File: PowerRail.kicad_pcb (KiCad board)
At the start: 2 copper layers, 25.4 x 25.4 mm, 20 parts, among them P1 PIN, P2 POUT, U1 ADP5071

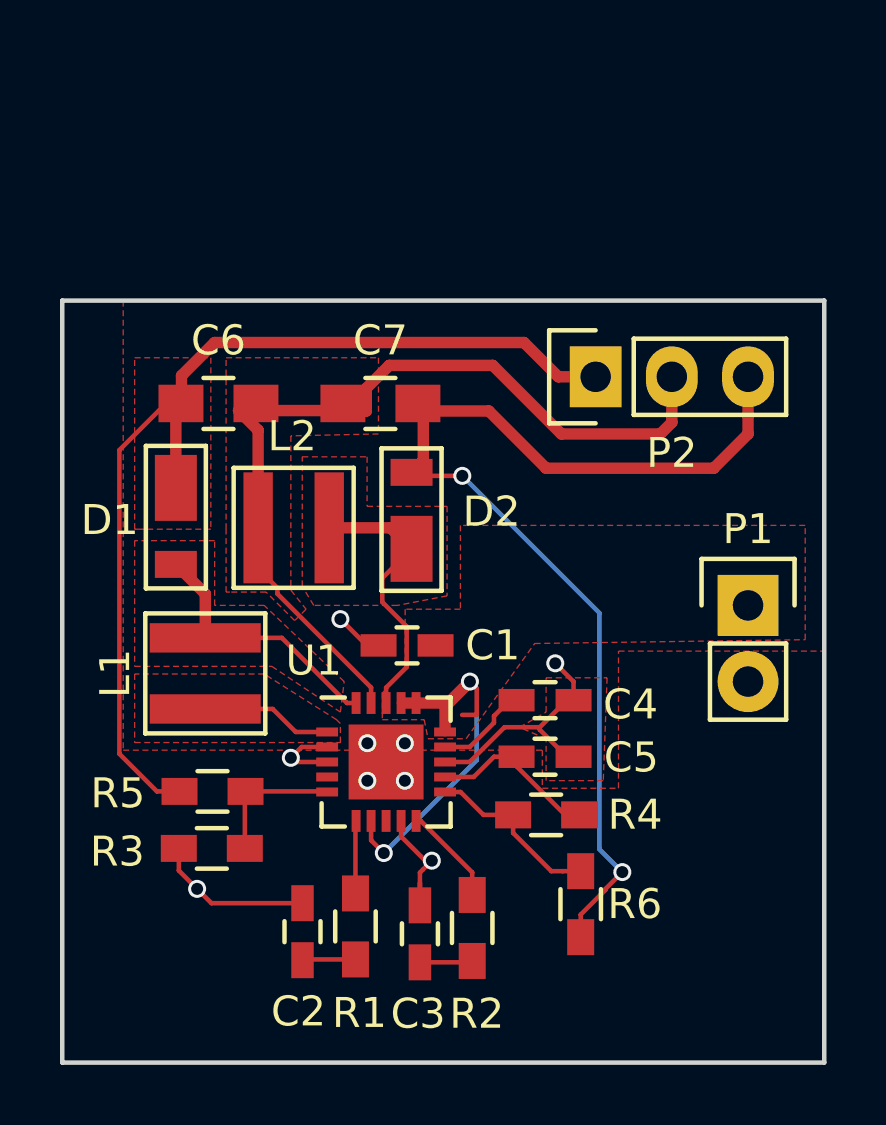
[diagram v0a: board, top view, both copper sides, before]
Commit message: Slight changes. Note: Need to add a net-tie
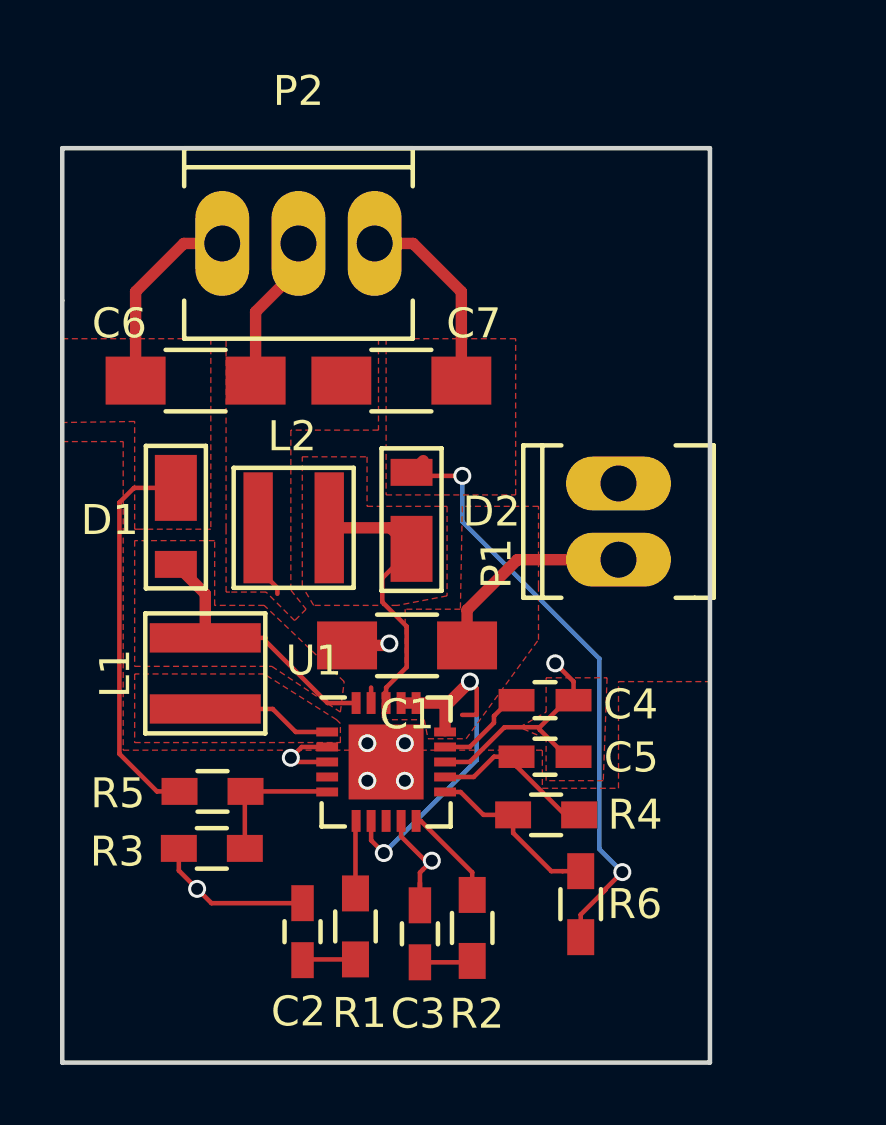
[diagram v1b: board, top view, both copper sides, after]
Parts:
- C1: value 10.0uF -> 22.0uF; footprint Capacitors_SMD:C_0603_HandSoldering -> Capacitors_SMD:C_1206_HandSoldering
- C6, C7: footprint Capacitors_SMD:C_0805_HandSoldering -> Capacitors_SMD:C_1206_HandSoldering
- P1: footprint Pin_Headers:Pin_Header_Straight_1x02 -> Sockets_MOLEX_KK-System:Socket_MOLEX-KK-RM2-54mm_Lock_2pin_straight
- P2: footprint Pin_Headers:Pin_Header_Straight_1x03 -> Sockets_MOLEX_KK-System:Socket_MOLEX-KK-RM2-54mm_Lock_3pin_straight
- R6: value 10.7M -> 1.07M
- moved P2 10.9 mm to (185.7, 74.3), turned to 0 degrees
- moved P1 5.14 mm to (196.3, 83.6), turned to 90 degrees
- moved C6 1.08 mm to (182.2, 78.9)
- moved C7 1.03 mm to (189.1, 78.9)
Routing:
- net /0V: track 29.7 -> 8.15 mm
- net /+12V: track 33.8 -> 19.5 mm
- net /-7V: track 36.4 -> 27.2 mm
- net +5V: track 13.4 -> 20.3 mm
- net (no net): track 1.66 -> 0.00 mm, vias 1 -> 0
- net GND: track 25.4 -> 26.9 mm, vias 8 -> 9
- added copper zone on F.Cu, net /-7V
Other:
- board size 25.4 x 25.4 mm -> 21.6 x 30.5 mm
